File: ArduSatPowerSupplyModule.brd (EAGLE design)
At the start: 95.5 x 90.3 mm, 168 parts, among them IC1 AVR-MEGA8-MI, IC11 MAX4372F, IC18 TMP102, IC19 TMP102, IC3 MAX17043G+U, IC7 MAX4372F, IC8 ATMEGA16U2-MU, J1 POWER_JACKPTH, P3 ICSP:USB, P4 microSD, Q1 RJU003N03 N-MOSFET, Q2 MOSFET-PCHANNELSMT2, Q3 RJU003N03 N-MOSFET, Q4 RJU003N03 N-MOSFET, Q43 RJU003N03 N-MOSFET, Q44 RJU003N03 N-MOSFET, Q45 RJU003N03 N-MOSFET, Q46 RJU003N03 N-MOSFET, Q5 RJU003N03 N-MOSFET, SW2 RESET

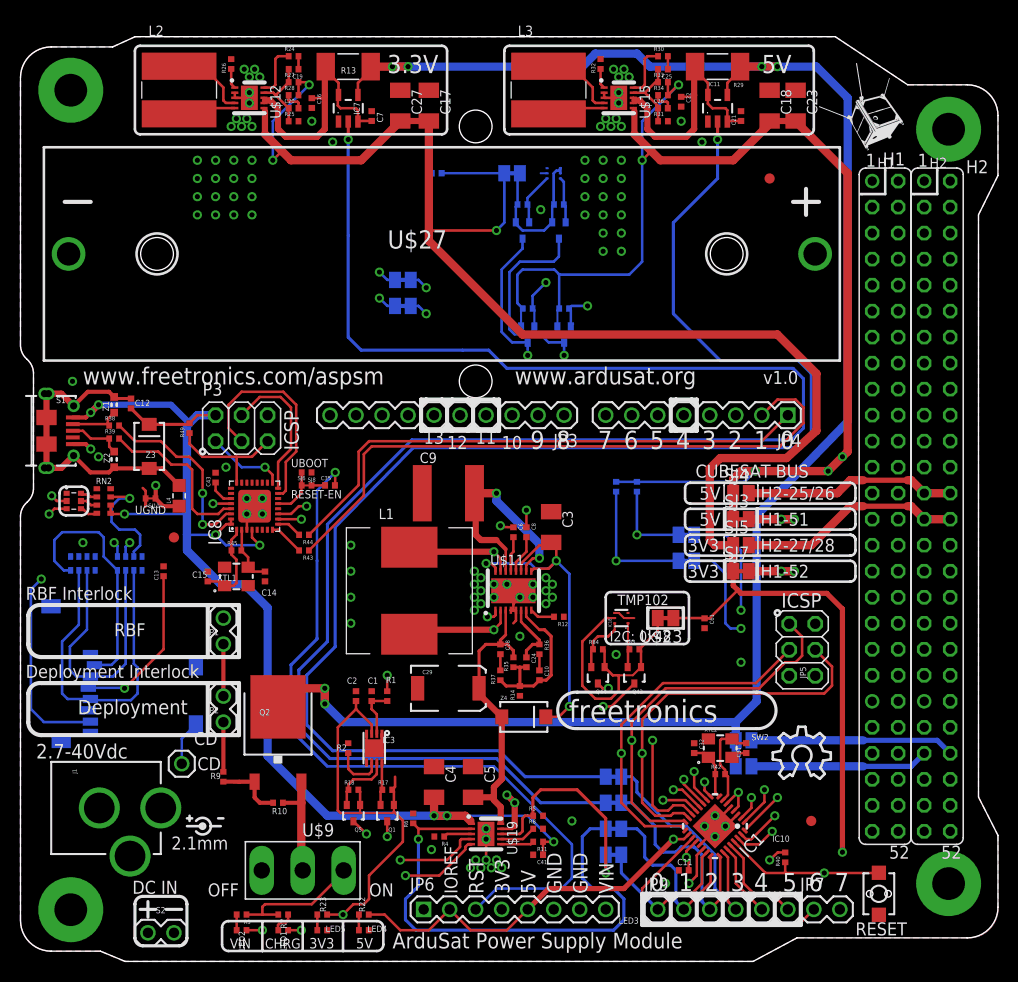
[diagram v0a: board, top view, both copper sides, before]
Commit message: Routing done, clearances, DRC, overlay. Nearly ready for v1.0 release
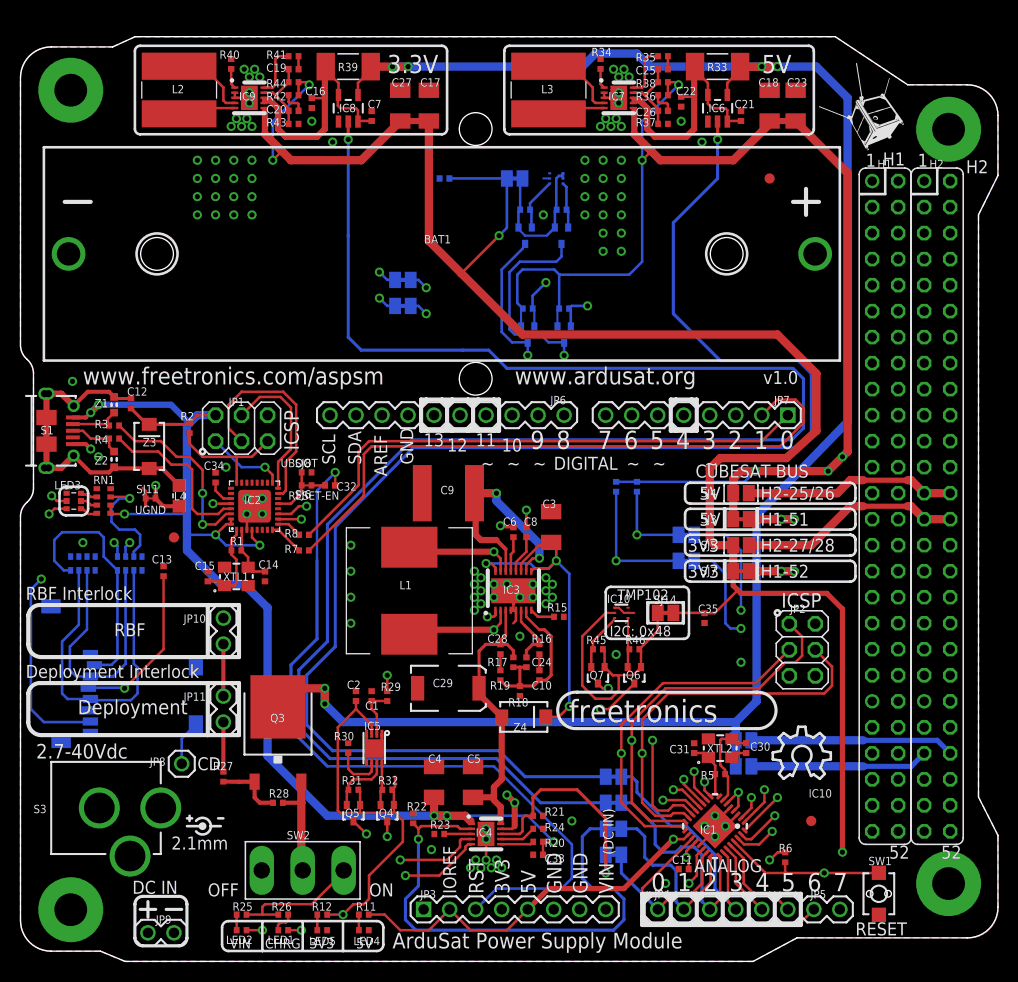
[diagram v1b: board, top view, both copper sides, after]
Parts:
- removed C61, C62: 100nF 0402, freetronics-jon:0402C
- removed IC18, IC19: TMP102, freetronics-jon:SOT563
- removed P3: ICSP:USB, pinhead:2X03
- removed P4: microSD, freetronics-master-v1:MICRO-SD-SOCKET-PP
- removed Q45, Q46: RJU003N03 N-MOSFET, freetronics-jon:SOT32-3
- removed R49, R84, R85, R86: 10K 0402, freetronics-jon:0402
- removed RN8: 2K2, freetronics-master-v1:CAY16
- removed U$11: LTC3115, freetronics-jon:DFN-16
- removed U$15: LTC3536, freetronics-jon:DFN-10
- removed U$23, U$24: SJCN, freetronics-jon:SJC
- removed U$9: SWITCH-SPDT, freetronics-jon:SS-12F100
- added C30: 22pF 0402, freetronics-jon:0402C
- added C36: 100nF 0402, freetronics-jon:0402C
- added IC10: TMP102, freetronics-jon:SOT563
- added IC2: ATMEGA16U2-MU, freetronics-jon:ATMEL_QFN32
- added IC5: MAX17043G+U, SparkFun:TDFN-8
- added IC6: MAX4372F, freetronics-jon:SOT23-5
- added JP10, JP11: (no value), freetronics-master-v1:1X02
- added Q8, Q9: RJU003N03 N-MOSFET, freetronics-jon:SOT32-3
- added R15: 121K 1% 0402, freetronics-jon:0402
- added R16: 93.1K 1% 0402, freetronics-jon:0402
- added R47, R48: 10K 0402, freetronics-jon:0402
- added RN1: 1K5, resistor-dil:CAY16
- added SJ14, SJ15: SJCN, freetronics-jon:SJC
- added SW1: RESET, freetronics-master-v1:TACTILE_SWITCH_SMD_2PIN_TINY
- C19: value 1nF -> 1nF 0402
- C2: value 10nF -> 10nF 0402
- C21, C33, C7: value 100nF 0603 -> 100nF 0402
- C26: value 100pF -> 100pF 0402
- C31: value 22pF 0603 -> 22pF 0402
- C32: value 22pF 0603 -> 100nF 0402
- IC11: value MAX4372F -> TMP102; device freetronics-jon:SOT23-5 -> freetronics-jon:SOT563
- IC3: value MAX17043G+U -> LTC3115; device SparkFun:TDFN-8 -> freetronics-jon:DFN-16
- IC7: value MAX4372F -> LTC3536; device freetronics-jon:SOT23-5 -> freetronics-jon:DFN-10
- IC8: value ATMEGA16U2-MU -> MAX4372F; device freetronics-jon:ATMEL_QFN32 -> freetronics-jon:SOT23-5
- JP1: value (none) -> ICSP:16U2; device freetronics-master-v1:1X02 -> pinhead:2X03
- JP2: value (none) -> ICSP:328P; device freetronics-master-v1:1X02 -> pinhead:2X03
- JP3: value M100.1 -> (none); device freetronics-marc:1X10 -> freetronics-marc:1X08
- JP4: device freetronics-marc:1X08 -> freetronics-marc:1X06
- JP5: value ICSP:MAIN -> (none); device pinhead:2X03 -> freetronics-marc:1X02
- JP6: value (none) -> M100.1; device freetronics-marc:1X08 -> freetronics-marc:1X10
- JP7: device freetronics-marc:1X02 -> freetronics-marc:1X08
- JP8: value M01PTH -> CD
- JP9: device freetronics-marc:1X06 -> freetronics-master-v1:1X02
- LED4: value BLUE -> BLUE 0402
- LED5: value JADEGREEN -> JADEGREEN 0402
- Q2: value MOSFET-PCHANNELSMT2 -> RJU003N03 N-MOSFET; device freetronics-jon:DPAK -> freetronics-jon:SOT32-3
- Q3: value RJU003N03 N-MOSFET -> MOSFET-PCHANNELSMT2; device freetronics-jon:SOT32-3 -> freetronics-jon:DPAK
- R1: value 1K -> 1M 0402
- R10: value 33K -> 10K 0402
- R11: value 1K -> 2K2 0402
- R12: value 121K 1% 0402 -> 1K 0402
- R13: value 0.1R 2010 -> 4K7 0402; device freetronics-original:R2010 -> freetronics-jon:0402
- R14: value 249K 1% 0402 -> 4K7 0402
- R17: value 10K 0402 -> 1M 1% 0402
- R18: value 10K 0402 -> 249K 1% 0402
- R19: value 4K7 0402 -> 249K 1% 0402
- R2: value 4K7 -> 10K 0402
- R20: value 10K 0402 -> 1K
- R21: value 10K 0402 -> 1.05K 1% 0603
- R22: value 2K2 -> 1.18K 1% 0603
- R23: value 1K -> 1K 1% 0402
- R24: value 49.9K -> 10K 0603
- R25: value 187K -> 2K2 0402
- R26: value 100K -> 1K 0402
- R27: value 845K -> 1K
- R28: value 15K -> 33K
- R29: value 0.1R 2010 -> 1K 0402; device freetronics-original:R2010 -> freetronics-jon:0402
- R3: value 2K2 -> 22R
- R30: value 49.9K -> 4K7 0402
- R31: value 115K -> 10K 0402
- R32: value 100K -> 10K 0402
- R33: value 845K -> 0.1R 2010; device freetronics-jon:0402 -> freetronics-original:R2010
- R34: value 15K -> 100K
- R35: value 1M 1% 0402 -> 49.9K
- R36: value 93.1K 1% 0402 -> 15K 0402
- R37: value 249K 1% 0402 -> 115K 1% 0402
- R38: value 22R -> 845K 1% 0402
- R39: value 22R -> 0.1R 2010; device freetronics-jon:0402 -> freetronics-original:R2010
- R4: value 1K 1% 0603 -> 22R
- R40: value 10K 0402 -> 100K
- R41: value 4K7 0402 -> 49.9K 1% 0402
- R42: value 1M 0402 -> 15K
- R43: value 1K 0402 -> 187K 1% 0402
- R44: value 1K 0402 -> 845K 1% 0402
- R45: value 1M 0402 -> 10K 0402
- R5: value 1.05K 1% 0603 -> 1M 0402
- R6: value 1.18K 1% 0603 -> 10K 0402
- R7: value 1K -> 1K 0402
- R8: value 10K 0603 -> 1K 0402
- R9: value 1K -> 10K 0402
- RN2: value 1K5 -> 2K2; device resistor-dil:CAY16 -> freetronics-master-v1:CAY16
- S2: value (none) -> microSD; device freetronics-master-v1:1X02 -> freetronics-master-v1:MICRO-SD-SOCKET-PP
- SW2: value RESET -> SWITCH-SPDT; device freetronics-master-v1:TACTILE_SWITCH_SMD_2PIN_TINY -> freetronics-jon:SS-12F100
- moved R40 94.5 mm to (20.6, 87.6)
- moved R26 83.2 mm to (25.7, 4.57), turned to 0 degrees
- moved R24 79.1 mm to (50.5, 13.0)
- moved R42 78.3 mm to (26.7, 84.6)
- moved R25 77.6 mm to (21.6, 4.57), turned to 180 degrees
- moved R30 74.2 mm to (32.0, 20.8), turned to 270 degrees
- moved R32 73.9 mm to (35.8, 16.8), turned to 0 degrees
- moved R31 71.9 mm to (32.5, 16.8)
- moved R29 69.4 mm to (35.8, 25.9), turned to 90 degrees
- moved R28 69.1 mm to (25.1, 15.5), turned to 180 degrees
- moved R27 68.2 mm to (19.8, 18.0), turned to 270 degrees
- moved R38 63.2 mm to (62.7, 85.9)
- moved R35 61.0 mm to (62.7, 88.4), turned to 0 degrees
- moved JP2 56.7 mm to (76.3, 30.4)
- moved SW2 56.3 mm to (27.6, 8.89), turned to 180 degrees
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- renumbered C41 to C33, C43 to C34, CD to JP8, J1 to S3, Q43 to Q6, Q44 to Q7, R83 to R46, RN6 to RN3, U$12 to IC9, U$14 to SJ19, U$19 to IC4, U$20 to SJ12, U$21 to SJ13, U$25 to SJ16, U$26 to SJ17, U$27 to BAT1, U$3 to SJ18
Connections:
- net 3.3V: now also C35.1, C36.1, IC5.3, JP3.4, Q4.1, R12.1, R31.2, R32.2, R42.2, R44.2, S2.4, SJ14.1, SJ15.1; no longer C61.1, C62.1, IC3.3, JP6.4, P4.4, Q1.1, R17.2, R18.2, R23.1, R27.2, R28.2, U$23.1, U$24.1
- net 3V3SENSED: now also IC8.3, IC8.5, R39.2; no longer IC7.3, IC7.5, R13.2
- net 5V: now also IC7.6, JP2.2, JP3.2, JP3.5, Q1.1, Q2.1, R10.2, R11.1, R13.2, R14.2, R36.2, R38.2, R6.2, R9.2; no longer JP5.2, JP6.2, JP6.5, Q3.1, Q4.1, R19.2, R20.2, R21.2, R22.1, R33.2, R34.2, R40.2, R41.2, U$15.6
- net 5VSENSED: now also IC6.3, IC6.5, IC7.7, IC7.8, R33.2; no longer IC11.3, IC11.5, R29.2, U$15.7, U$15.8
- net A0: now also JP4.1; no longer JP9.1
- net A1: now also JP4.2; no longer JP9.2
- net A2: now also JP4.3; no longer JP9.3
- net A3: now also JP4.4; no longer JP9.4
- net A4_SDA: now also JP4.5, JP6.9; no longer JP3.9, JP9.5
- net A5_SCL: now also JP4.6, JP6.10; no longer JP3.10, JP9.6
- net A6: now also JP5.1; no longer JP7.1
- net A7: now also JP5.2; no longer JP7.2
- net AREF: now also JP6.8; no longer JP3.8
- net BAT: now also R25.1, R26.1, R29.2, SW2.1; no longer R1.2, R3.1, R7.1, U$9.1
- net CELL: now also IC5.2, R29.1; no longer IC3.2, R1.1
- net D+: now also R4.1; no longer R39.1
- net D-: now also R3.1; no longer R38.1
- net D0_RX: now also JP7.1, R8.1; no longer JP4.1, R44.1
- net D10: now also JP6.3; no longer JP3.3
- net D11_MOSI: now also JP2.4, JP6.4; no longer JP3.4, JP5.4
- net D12_MISO: now also JP2.1, JP6.5, S2.7; no longer JP3.5, JP5.1, P4.7
- net D13_SCK: now also JP2.3, JP6.6, RN1.3; no longer JP3.6, JP5.3, RN2.3
- net D1_TX: now also JP7.2, R7.1; no longer JP4.2, R43.1
- net D2_SDA: now also JP7.3; no longer JP4.3
- net D3_SCL: now also JP7.4; no longer JP4.4
- net D4: now also JP7.5; no longer JP4.5
- net D5: now also JP7.6; no longer JP4.6
- net D6: now also JP7.7; no longer JP4.7
- net D7: now also JP7.8; no longer JP4.8
- net D8: now also JP6.1; no longer JP3.1
- net D9: now also JP6.2; no longer JP3.2
- net DC_I: now also R21.1; no longer R5.1
- net DTR: now also IC2.13; no longer IC8.13
- net GND: now also C30.1, C35.2, C36.2, IC10.2, IC10.4, IC11.2, IC2.3, IC2.EXP, IC3.5, IC3.TGND, IC5.1, IC5.4, IC5.EP, IC6.1, IC7.2, IC7.3, IC7.TGND, IC8.1, JP1.6, JP10.1, JP2.6, JP3.6, JP9.1, R15.1, R18.1, R21.2, R22.2, R23.2, R24.2, R30.1, R34.2, R37.2, R40.2, R43.2, RN2.1, RN2.2, RN2.3, S2.6, S2.CD2, S2.GND1, S2.GND2, SW1.1; no longer C32.1, C61.2, C62.2, IC11.1, IC18.2, IC18.4, IC19.2, IC3.1, IC3.EP, IC7.1, IC8.3, IC8.EXP, JP1.1, JP5.6, JP6.6, P3.6, P4.6, P4.CD2, P4.GND1, P4.GND2, R12.1, R14.1, R2.1, R25.2, R26.2, R31.2, R32.2, R4.2, R5.2, R6.2, R8.2, RN8.1, RN8.2, RN8.3, S2.1, SW2.1, U$11.4, U$11.5, U$11.TGND, U$15.2, U$15.3, U$15.TGND
- net MISO2: now also IC2.17, JP1.1; no longer IC8.17, P3.1
- net MOSI2: now also IC2.16, JP1.4; no longer IC8.16, P3.4
- net N$1: now also R12.2; no longer R23.2
- net N$10: now also C30.2, R5.2; no longer C31.2, R42.2
- net N$10001: now also IC10.6, R45.1; no longer IC18.6, R84.1
- net N$10002: now also IC11.6, Q9.2, R47.1; no longer IC19.6, Q46.2, R86.1
- net N$10003: now also IC11.1, Q8.2, R48.1; no longer IC19.1, Q45.2, R85.1
- net N$11: now also IC6.2; no longer IC11.2
- net N$12: now also IC2.1, R1.1; no longer IC8.1, R45.1
- net N$13: now also RN2.8, S2.2; no longer P4.2, RN8.8
- net N$14: now also RN1.6; no longer RN2.6
- net N$15: now also R41.1; no longer R24.1
- net N$16: now also RN1.7; no longer RN2.7
- net N$17: now also RN1.8; no longer RN2.8
- net N$2: now also JP10.2, JP11.1; no longer JP1.2, JP2.1
- net N$20: now also R24.1; no longer R8.1
- net N$21: now also R40.1; no longer R26.1
- net N$22: now also IC7.4; no longer U$15.4
- net N$23: now also R41.2; no longer R24.2
- net N$24: now also C31.2, R5.1; no longer C32.2, R42.1
- net N$248: now also R26.2; no longer R7.2
- net N$25: now also R42.1; no longer R28.1
- net N$26: now also R43.1, R44.1; no longer R25.1, R27.1
- net N$28: now also IC7.5; no longer U$15.5
- net N$29: now also IC7.1, R34.1; no longer R32.1, U$15.1
- net N$3: now also R25.2; no longer R3.2
- net N$30: now also R35.2; no longer R30.2
- net N$31: now also IC7.10, R35.1; no longer R30.1, U$15.10
- net N$32: now also R36.1; no longer R34.1
- net N$33: now also IC7.9, R37.1, R38.1; no longer R31.1, R33.1, U$15.9
- net N$34: now also IC2.27; no longer IC8.27
- net N$35: now also R23.1; no longer R4.1
- net N$36: now also R20.2; no longer R11.2
- net N$37: now also R16.2; no longer R36.2
- net N$39: now also IC3.11, IC3.16, IC3.9; no longer U$11.11, U$11.16, U$11.9
- net N$4: now also JP11.2, R27.1; no longer JP2.2, R9.1
- net N$40: now also IC3.13; no longer U$11.13
- net N$41: now also IC3.12; no longer U$11.12
- net N$42: now also IC3.15; no longer U$11.15
- net N$43: now also IC3.2; no longer U$11.2
- net N$44: now also IC3.6, R16.1; no longer R36.1, U$11.6
- net N$45: now also IC3.7, R17.1, R18.2, R19.1; no longer R14.2, R35.1, R37.1, U$11.7
- net N$46: now also RN2.6, S2.3; no longer P4.3, RN8.6
- net N$47: now also IC3.8, R15.2; no longer R12.2, U$11.8
- net N$48: now also RN2.7, S2.5; no longer P4.5, RN8.7
- net N$49: now also R19.2; no longer R37.2
- net N$5: now also Q3.3, R28.1, SW2.2; no longer Q2.3, R10.1, U$9.2
- net N$50: now also S2.CD1; no longer P4.CD1
- net N$51: now also IC8.2; no longer IC7.2
- net N$52: now also IC2.2, R1.2; no longer IC8.2, R45.2
- net N$53: now also IC10.5, R45.2, SJ14.2; no longer IC18.5, R84.2, U$23.2
- net N$54: now also IC11.4, IC11.5, Q8.1, Q9.1, R47.2, R48.2, SJ15.2; no longer IC19.4, IC19.5, Q45.1, Q46.1, R85.2, R86.2, U$24.2
- net N$55: now also Q1.2, R9.1; no longer Q3.2, R20.1
- net N$56: now also IC2.28; no longer IC8.28
- net N$57: now also Q2.2, R10.1; no longer Q4.2, R21.1
- net N$6: now also R11.2; no longer R22.2
- net N$60: now also C32.1; no longer C35.1
- net N$7: now also Q3.1, R27.2, R28.2; no longer Q2.1, R10.2, R9.2
- net N$8: now also IC5.8, Q4.2, R32.1; no longer IC3.8, Q1.2, R17.1
- net N$9: now also IC5.7, R31.1; no longer IC3.7, R18.1
- net N$9999: now also IC10.1; no longer IC18.1
- net NC: now also JP3.1; no longer JP6.1
- net PVIN: now also IC3.1, IC3.10, IC3.14, JP3.8, JP9.2; no longer JP6.8, S2.2, U$11.1, U$11.10, U$11.14
- net PVOUT: now also IC3.3, R17.2; no longer R35.2, U$11.3
- net QST: now also IC5.6, R30.2; no longer IC3.6, R2.2
- net RD+: now also IC2.29, R4.2; no longer IC8.29, R39.2
- net RD-: now also IC2.30, R3.2; no longer IC8.30, R38.2
- net RESET: now also C32.2, JP2.5, JP3.3, R6.1, SW1.2; no longer C35.2, JP5.5, JP6.3, R40.1, SW2.2
- net RESET2: now also IC2.24, JP1.5, R2.1; no longer IC8.24, P3.5, R49.1
- net RXLED: now also IC2.10; no longer IC8.10
- net SCK2: now also IC2.15, JP1.3; no longer IC8.15, P3.3
- net SCL: now also Q1.3, Q8.3, R13.1; no longer Q3.3, Q45.3, R41.1
- net SDA: now also Q2.3, Q9.3, R14.1; no longer Q1.3, Q46.3, R19.1
- net TXLED: now also IC2.11; no longer IC8.11
- net USBRXD: now also IC2.9, R8.2; no longer IC8.9, R44.2
- net USBTXD: now also IC2.8, R7.2; no longer IC8.8, R43.2
- net USBVCC: now also IC2.31, IC2.32, IC2.4, JP1.2, R2.2, R20.1, RN1.1, RN1.2; no longer IC8.31, IC8.32, IC8.4, P3.2, R11.1, R49.2, RN2.1, RN2.2
- net USB_I: now also R22.1; no longer R6.1
- net VBATT: now also IC6.4, IC8.4, Q3.2, R33.1, R39.1; no longer IC11.4, IC7.4, Q2.2, R13.1, R29.1
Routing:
- net 3.3V: track 351.2 -> 349.1 mm
- net N$53: track 26.0 -> 27.0 mm
- net N$9999: track 4.44 -> 4.95 mm
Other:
- board text added: "(DC IN)"
- board text added: "ANALOG"
- board text added: "AREF"
- board text added: "CUBESAT BUS H1-41: SDA H1-43: SCL H2-25: 5V H2-26: 5V H2-27: 3V3 H2-28: 3V3 H2-29: GND H2-30: GND H2-32: GND H2-45: VBATT45 H2-46: VBATT46"
- board text added: "DIGITAL"
- board text added: "I2C ADDRESSES 0x36: MAX17043G+U 0x48: TMP102 (TOP) 0x49: TMP102 (BOT)"
- board text added: "SW1"
- board text added: "~"
- board text removed: "H1-41: SDA H1-43: SCL H2-25: 5V H2-26: 5V H2-27: 3V3 H2-28: 3V3 H2-29: GND H2-30: GND H2-32: GND H2-45: VBATT45 H2-46: VBATT46"
- board text removed: "SW2"
- board text removed: "TEMP SENSOR I2C ADDRESSES TOP: 0x48 BOT: 0x49"
